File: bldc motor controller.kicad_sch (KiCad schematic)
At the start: 43 parts, among them SW1 SW_Push, SW2 SW_Push

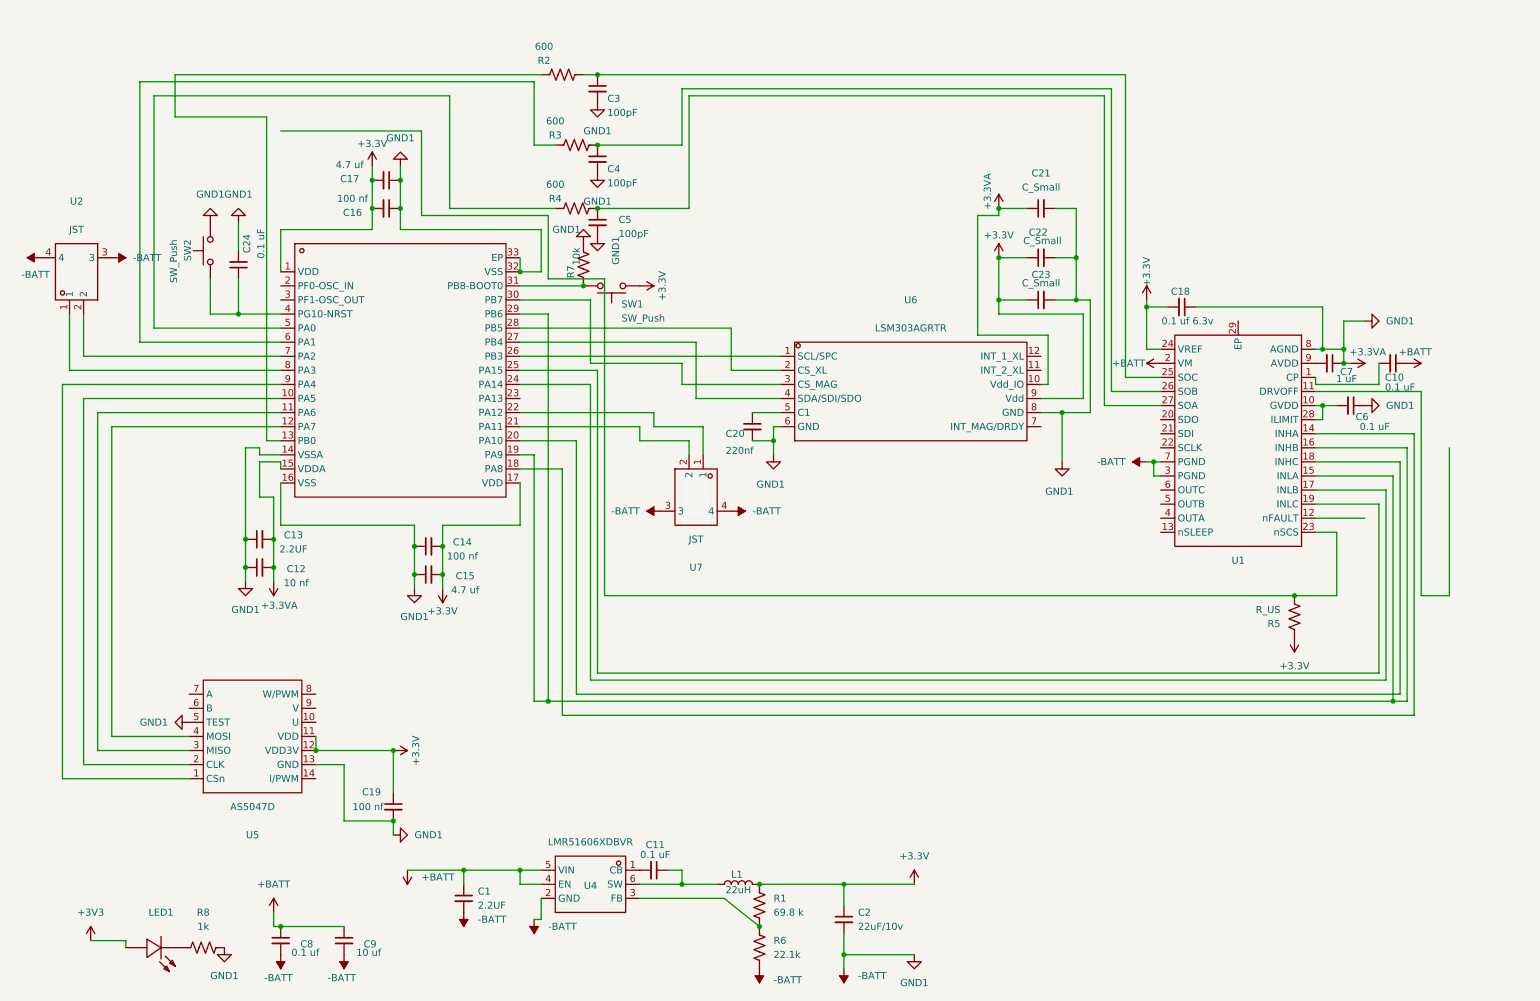
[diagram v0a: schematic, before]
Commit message: fuck yeah is closing in
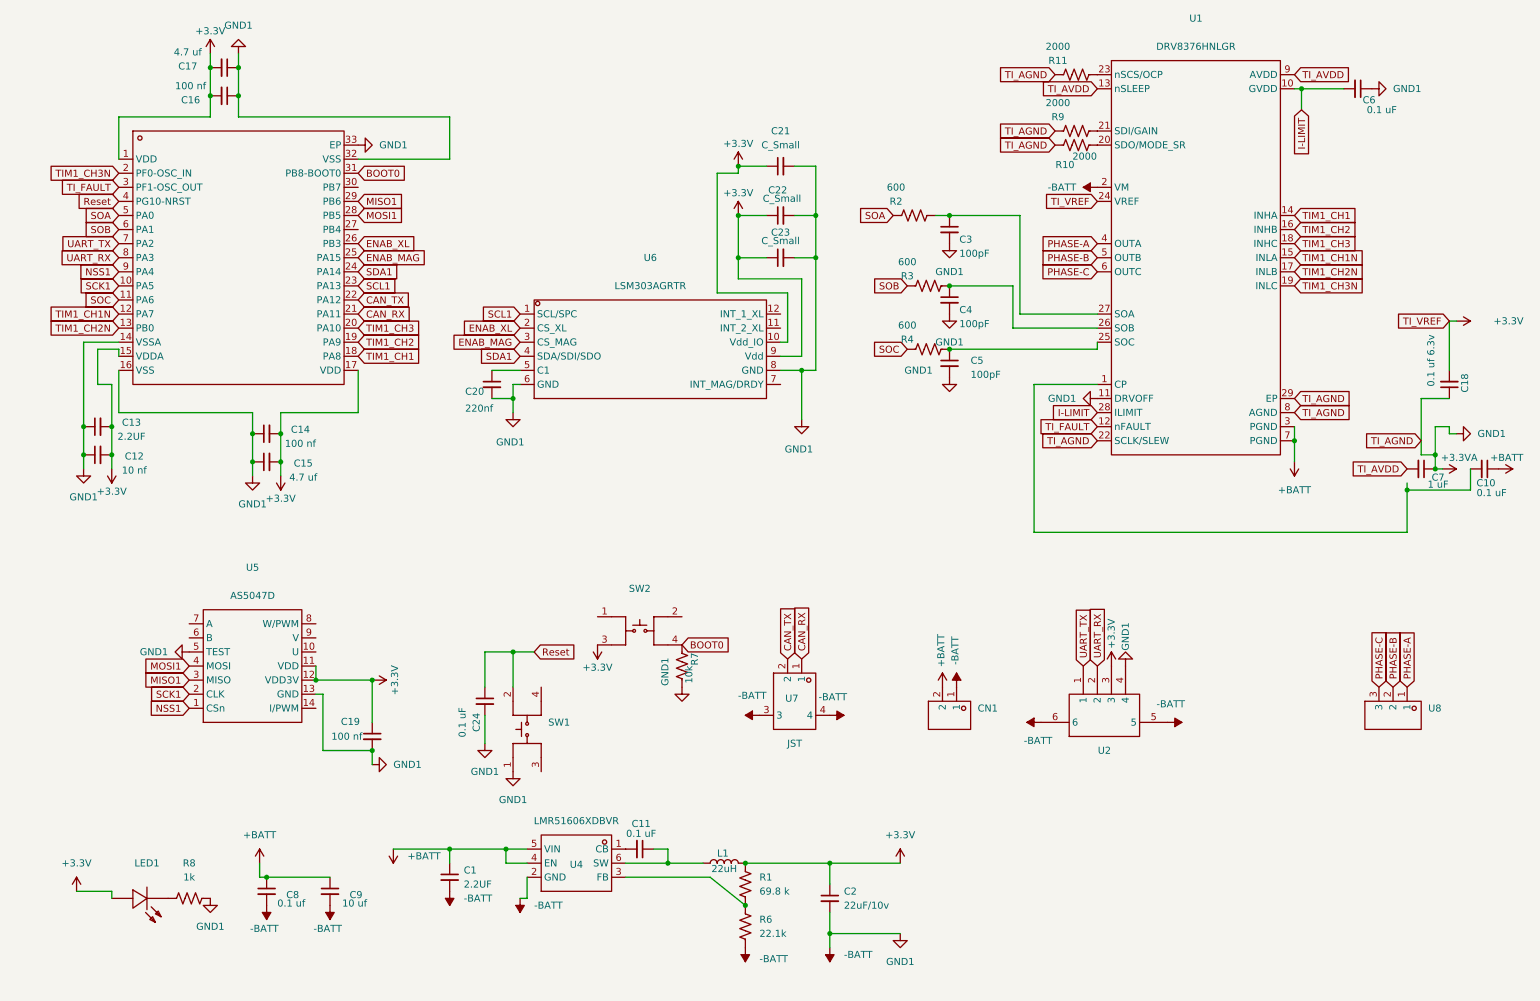
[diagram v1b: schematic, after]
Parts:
- removed R5: R_US, symbol Device:R_US
- removed SW1, SW2: SW_Push, symbol Switch:SW_Push
- removed U1: ~, ProLib_pcs_2025-09-24:VQFN-28_L6.0-W5.0-P0.50-TL-EP4.0, symbol bldc controller:DRV8376SNLGR
- removed U2: ~, ProLib_pcs_2025-10-01 (1):CONN-SMD_SM02B-GHS-TB-LF-SN, symbol bldc controller:SM02B-GHS-TB(LF)(SN)
- added CN1: ~, Connector_JST:JST_EH_B2B-EH-A_1x02_P2.50mm_Vertical, symbol bldc controller:WAFER-XH254WZ-2AM
- added R10, R11, R9: 2000, Resistor_SMD:R_01005_0402Metric, symbol Device:R_US
- added SW1, SW2: ~, bldc-motor-footprints:KEY-SMD_4P-L2.6-W1.6-P0.80-LS3.0, symbol bldc controller:SKTAACE010
- added U1: ~, bldc-motor-footprints:VQFN-28_L6.0-W5.0-P0.50-TL-EP4.0, symbol bldc controller:DRV8376HNLGR
- added U2: ~, bldc-motor-footprints:CONN-SMD_4P-P1.25_SM04B-GHS-TB-LF-SN, symbol bldc controller:SM04B-GHS-TB(LF)(SN)
- added U8: ~, Button_Switch_THT:SW_Slide-03_Wuerth-WS-SLTV_10x2.5x6.4_P2.54mm, symbol bldc controller:MR30-M
- C1: footprint (none) -> Capacitor_SMD:C_1206_3216Metric
- C10, C11, C18, C19, C24, C8: footprint (none) -> Capacitor_SMD:C_0402_1005Metric
- C12, C13, C14, C15, C16, C17, C20, C21, C22, C23, C3, C4, C5, C6: footprint (none) -> Capacitor_SMD:C_01005_0402Metric
- C2, R1: footprint (none) -> Capacitor_SMD:C_0805_2012Metric
- C7, C9: footprint (none) -> Capacitor_SMD:C_0603_1608Metric
- L1: footprint (none) -> Inductor_SMD:L_Bourns_SRP5030T
- LED1: footprint ProLib_pcs_2025-10-01 (3):LED0603-RD -> bldc-motor-footprints:LED0603-RD
- R2, R3, R4: footprint (none) -> Resistor_SMD:R_01005_0402Metric
- R6, R8: footprint (none) -> Resistor_SMD:R_0603_1608Metric
- R7: footprint (none) -> Resistor_SMD:R_0402_1005Metric
- U3: footprint ProLib_pcs_2025-10-01:QFN-32_L5.0-W5.0-P0.50-BL-EP3.7 -> bldc-motor-footprints:QFN-32_L5.0-W5.0-P0.50-BL-EP3.7
- U4: footprint 48v-3.3v buck:SOT-23-6_L2.9-W1.6-P0.95-LS2.8-BR -> bldc-motor-footprints:SOT-23-6_L2.9-W1.6-P0.95-LS2.8-BR
- U5: footprint ProLib_pcs_2025-10-01:TSSOP-14_L5.0-W4.4-P0.65-LS6.4-BL -> bldc-motor-footprints:TSSOP-14_L5.0-W4.4-P0.65-LS6.4-BL
- U6: footprint ProLib_pcs_2025-10-01 (2):LGA-12_L2.0-W2.0-P0.50-BL -> bldc-motor-footprints:LGA-12_L2.0-W2.0-P0.50-BL
- U7: footprint ProLib_pcs_2025-10-01 (1):CONN-SMD_SM02B-GHS-TB-LF-SN -> bldc-motor-footprints:CONN-SMD_SM02B-GHS-TB-LF-SN
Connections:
- net +3V3 is gone; now on net +3.3V: LED1.2 (A)
- net +3.3V: now also C12.2, C13.2, C21.1, U3.15 (VDDA), U6.10 (Vdd_IO), SW2.3, U1.24 (VREF), U2.3
- net +3.3VA: now also CN1.1, R10.2, R11.2, R9.2, SW1.1, U1.11 (DRVOFF), U1.2 (VM), U1.22 (SCLK/SLEW), U1.29 (EP), U1.8 (AGND), U2.4, U2.5, U2.6; no longer C12.2, C13.2, C21.1, U3.15 (VDDA), U6.10 (Vdd_IO)
- net +BATT: now also CN1.2, U1.3 (PGND), U1.7 (PGND)
- net at C3.1, R2.1: now also U1.27 (SOA)
- net SOA: now reaches R2.2
- net SOA: now also U3.5 (PA0); no longer U3.13 (PB0)
- net at C4.1, R3.1: now also U1.26 (SOB)
- net SOB: now reaches R3.2, U3.6 (PA1)
- net ENAB_XL: now reaches U3.26 (PB3)
- net ENAB_XL: now also U6.2 (CS_XL); no longer U6.1 (SCL/SPC)
- net MOSI1: now reaches U3.28 (PB5)
- net MOSI1: now also U5.4 (MOSI); no longer U6.2 (CS_XL)
- net at U3.30 (PB7): no longer U6.3 (CS_MAG)
- net at U3.27 (PB4): no longer U6.4 (SDA/SDI/SDO)
- net NSS1: now reaches U3.9 (PA4), U5.1 (CSn)
- net SCK1: now reaches U3.10 (PA5), U5.2 (CLK)
- net MISO1: now reaches U5.3 (MISO)
- net MISO1: now also U3.29 (PB6); no longer U3.11 (PA6)
- net TIM1_CH1N: now reaches U3.12 (PA7)
- net TIM1_CH1N: now also U1.15 (INLA); no longer U5.4 (MOSI)
- net TI_AVDD: now reaches C7.2
- net TI_AVDD: now also U1.13 (nSLEEP), U1.9 (AVDD)
- net Reset: now reaches C24.1, U3.4 (PG10-NRST)
- net Reset: now also SW1.2
- net CAN_RX: now reaches U7.1
- net CAN_RX: now also U3.21 (PA11); no longer U3.22 (PA12)
- net CAN_TX: now reaches U7.2
- net CAN_TX: now also U3.22 (PA12); no longer U3.21 (PA11)
- net at C10.2: now also U1.1 (CP)
- net I-LIMIT: now reaches C6.2
- net I-LIMIT: now also U1.10 (GVDD), U1.28 (ILIMIT)
- net TIM1_CH1: now reaches U3.18 (PA8)
- net TIM1_CH1: now also U1.14 (INHA)
- net TIM1_CH2: now reaches U3.19 (PA9)
- net TIM1_CH2: now also U1.16 (INHB); no longer U3.29 (PB6)
- net SDA1: now reaches U3.24 (PA14)
- net SDA1: now also U6.4 (SDA/SDI/SDO)
- net TIM1_CH3: now reaches U3.20 (PA10)
- net TIM1_CH3: now also U1.18 (INHC)
- net ENAB_MAG: now reaches U3.25 (PA15)
- net ENAB_MAG: now also U6.3 (CS_MAG)
- net at C5.1, R4.1: now also U1.25 (SOC)
- net UART_RX: now reaches U3.8 (PA3)
- net UART_RX: now also U2.2
- net UART_TX: now reaches U3.7 (PA2)
- net UART_TX: now also U2.1
- net TIM1_CH3N: now reaches U3.2 (PF0-OSC_IN)
- net TIM1_CH3N: now also U1.19 (INLC)
- net SCL1: now reaches U3.23 (PA13)
- net SCL1: now also U6.1 (SCL/SPC)
- net TI_FAULT: now reaches U3.3 (PF1-OSC_OUT)
- net TI_FAULT: now also U1.12 (nFAULT)
- net BOOT0: now reaches R7.1, U3.31 (PB8-BOOT0)
- net BOOT0: now also SW2.4
- net SOC: now reaches R4.2
- net SOC: now also U3.11 (PA6); no longer U3.5 (PA0)
- new net: R9.1, U1.21 (SDI/GAIN)
- new net: R10.1, U1.20 (SDO/MODE_SR)
- new net: R11.1, U1.23 (nSCS/OCP)
- new net PHASE-A: U1.4 (OUTA), U8.1
- new net PHASE-B: U1.5 (OUTB), U8.2
- new net PHASE-C: U1.6 (OUTC), U8.3
- new net TIM1_CH2N: U1.17 (INLB), U3.13 (PB0)
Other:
- moved on the sheet: C1, C10, C11, C12, C13, C14, C15, C16, C17, C18, C19, C2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
